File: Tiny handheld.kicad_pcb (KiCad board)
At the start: 2 copper layers, 34.3 x 58.4 mm, 38 parts, among them J1 Conn_01x04_Female, J3 TYPE-C-31-M-12, U1 ATtiny85-20P, U2 ATtiny85-20M, U3 EEPROM-I2CEIAJ

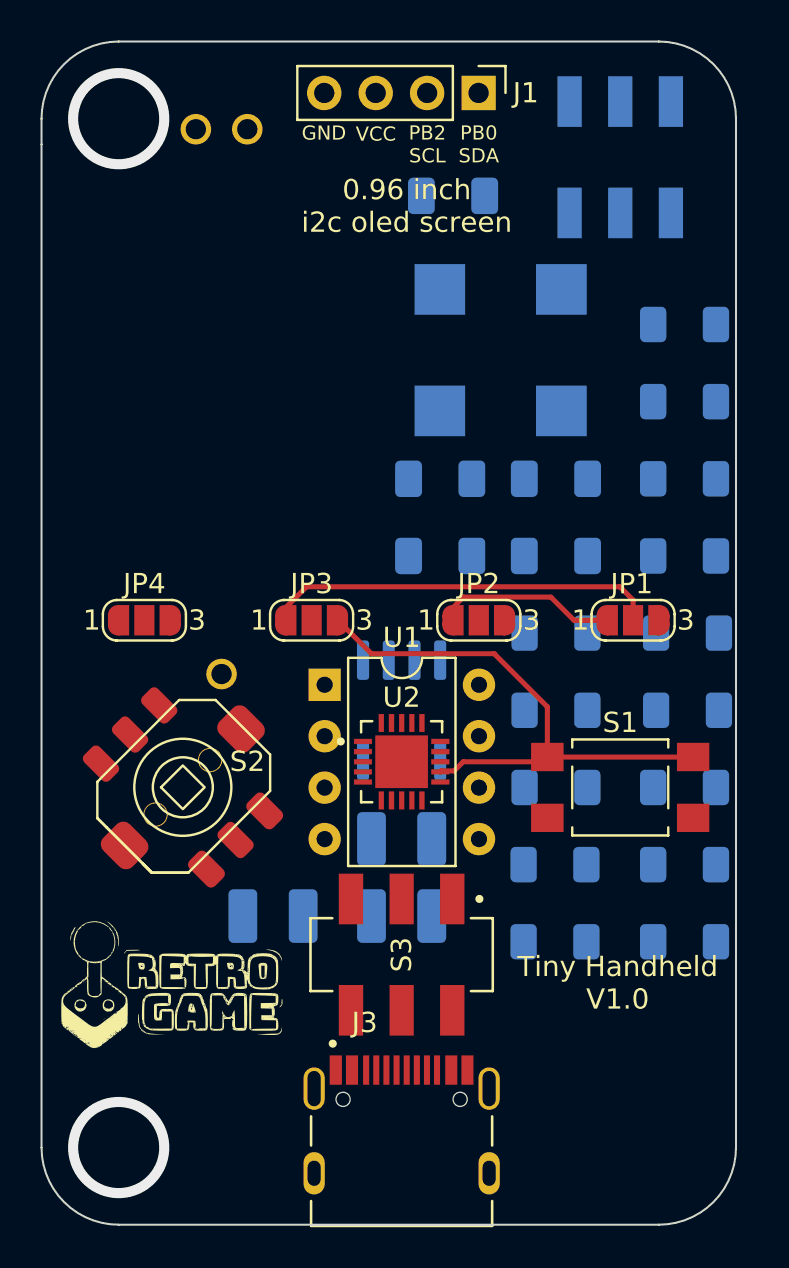
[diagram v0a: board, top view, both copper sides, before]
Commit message: continued wiring
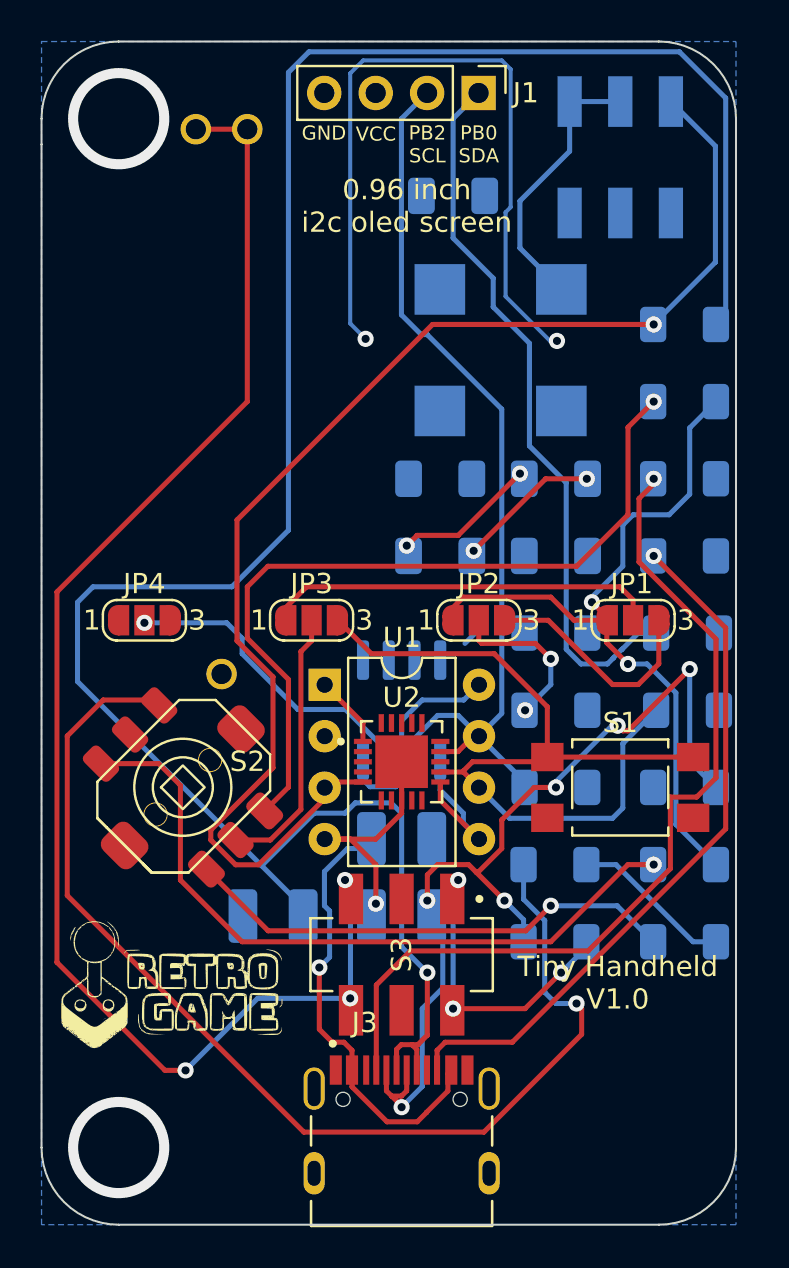
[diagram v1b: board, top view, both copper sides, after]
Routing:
- net Net-(D2-Pad1): track 0.00 -> 113.0 mm, vias 0 -> 1
- net Net-(BT1-Pad+): track 0.00 -> 71.7 mm, vias 0 -> 3
- net PB4: track 0.00 -> 65.6 mm, vias 0 -> 1
- net Net-(R1-Pad2): track 0.00 -> 55.7 mm, vias 0 -> 1
- net PB2/SCL/SCK: track 0.00 -> 45.8 mm
- net Net-(D3-Pad1): track 0.00 -> 45.3 mm, vias 0 -> 6
- net PB0/SDA/MOSI: track 0.00 -> 44.9 mm
- net Net-(J3-PadA5): track 0.00 -> 43.9 mm, vias 0 -> 1
- net Net-(R4-Pad2): track 0.00 -> 38.8 mm, vias 0 -> 1
- net (no net): track 0.00 -> 36.6 mm, vias 2 -> 4
- net Net-(R7-Pad2): track 0.00 -> 35.3 mm, vias 0 -> 1
- net Net-(J3-PadB5): track 0.00 -> 34.7 mm, vias 0 -> 1
- net Net-(JP1-Pad1): track 8.92 -> 38.4 mm, vias 0 -> 2
- net Net-(R3-Pad2): track 0.00 -> 24.6 mm, vias 0 -> 1
- net Net-(D1-Pad2): track 0.00 -> 22.1 mm, vias 0 -> 1
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- added copper zone on B.Cu, net GND

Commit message: more connections made
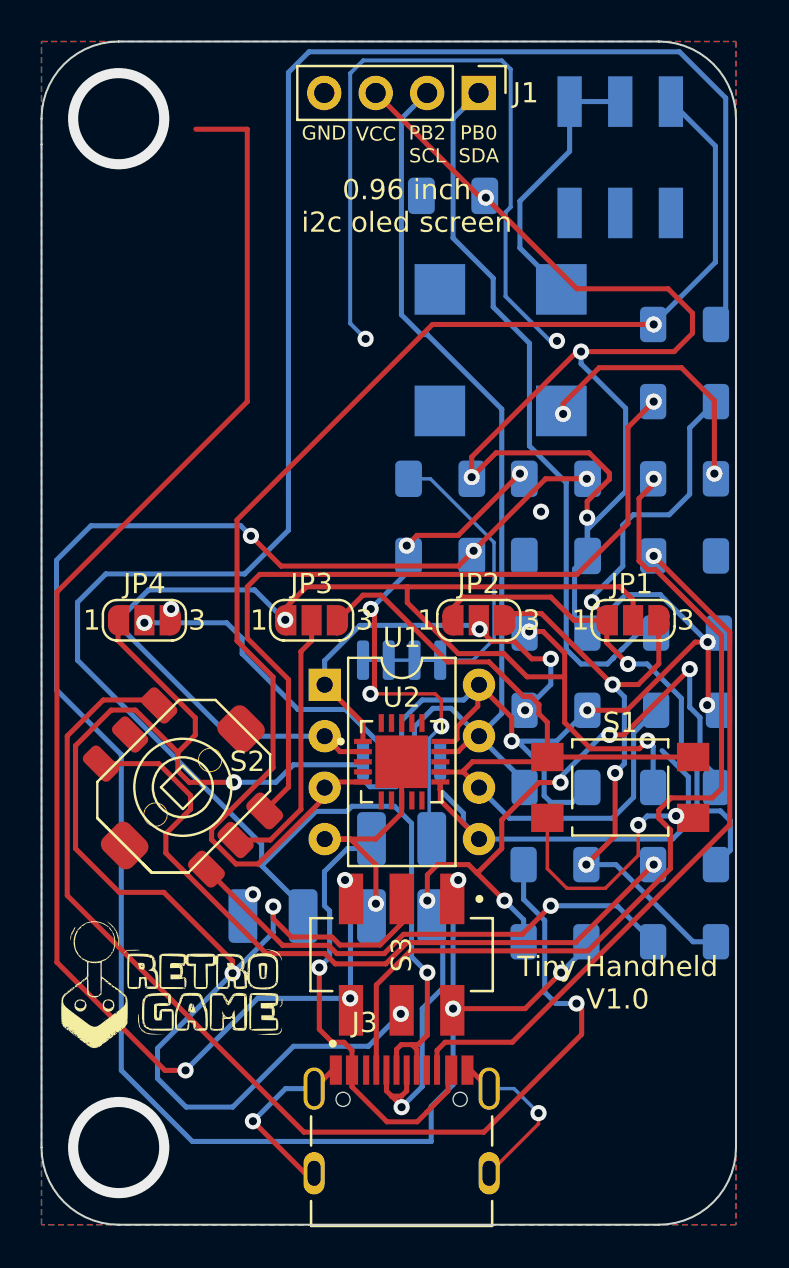
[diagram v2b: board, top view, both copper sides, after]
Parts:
- removed BT1: BATTERY-6.8MM_SMD, Snapeda:BAT_BU2032-1
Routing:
- net VCC: track 10.7 -> 186.9 mm, vias 0 -> 12
- net ExtVCC: track 21.6 -> 94.3 mm, vias 5 -> 6
- net GND: track 11.9 -> 72.5 mm, vias 1 -> 10
- net PB3: track 19.5 -> 66.4 mm, vias 0 -> 3
- net Net-(C1-Pad2): track 7.06 -> 26.5 mm, vias 2 -> 5
- net PB0/SDA/MOSI: track 44.9 -> 59.7 mm
- net Net-(JP1-Pad3): track 19.5 -> 29.7 mm, vias 0 -> 3
- net PB5/RES: track 13.0 -> 21.3 mm, vias 2 -> 3
- net Net-(R7-Pad2): track 35.3 -> 36.8 mm
- net Net-(J3-PadA5): track 43.9 -> 45.3 mm
- net Net-(JP1-Pad1): track 38.4 -> 39.5 mm
- net Net-(R3-Pad2): track 24.6 -> 25.5 mm
- net PB1/MISO: track 42.0 -> 42.8 mm
- net PB2/SCL/SCK: track 45.8 -> 46.5 mm
- added copper zone on F.Cu, net GND
